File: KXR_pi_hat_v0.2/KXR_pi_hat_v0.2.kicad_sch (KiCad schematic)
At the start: 6 parts, among them J1 Conn_01x05_Pin, J2 Conn_01x05_Pin, J3 Conn_01x05_Pin, J4 Conn_01x05_Pin, U2 Raspberry_Pi_2_3

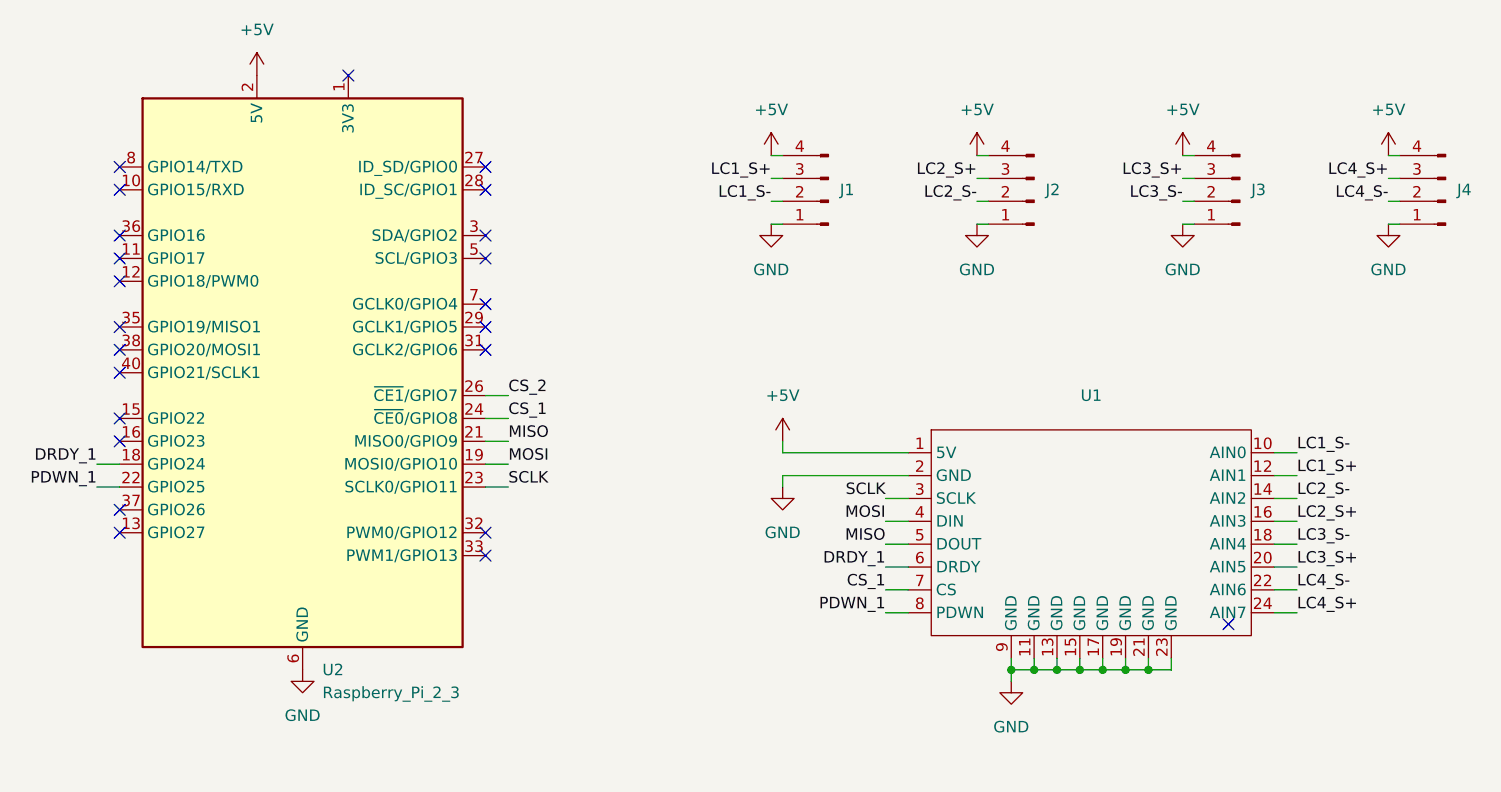
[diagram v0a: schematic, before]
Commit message: Finishing touches and production files
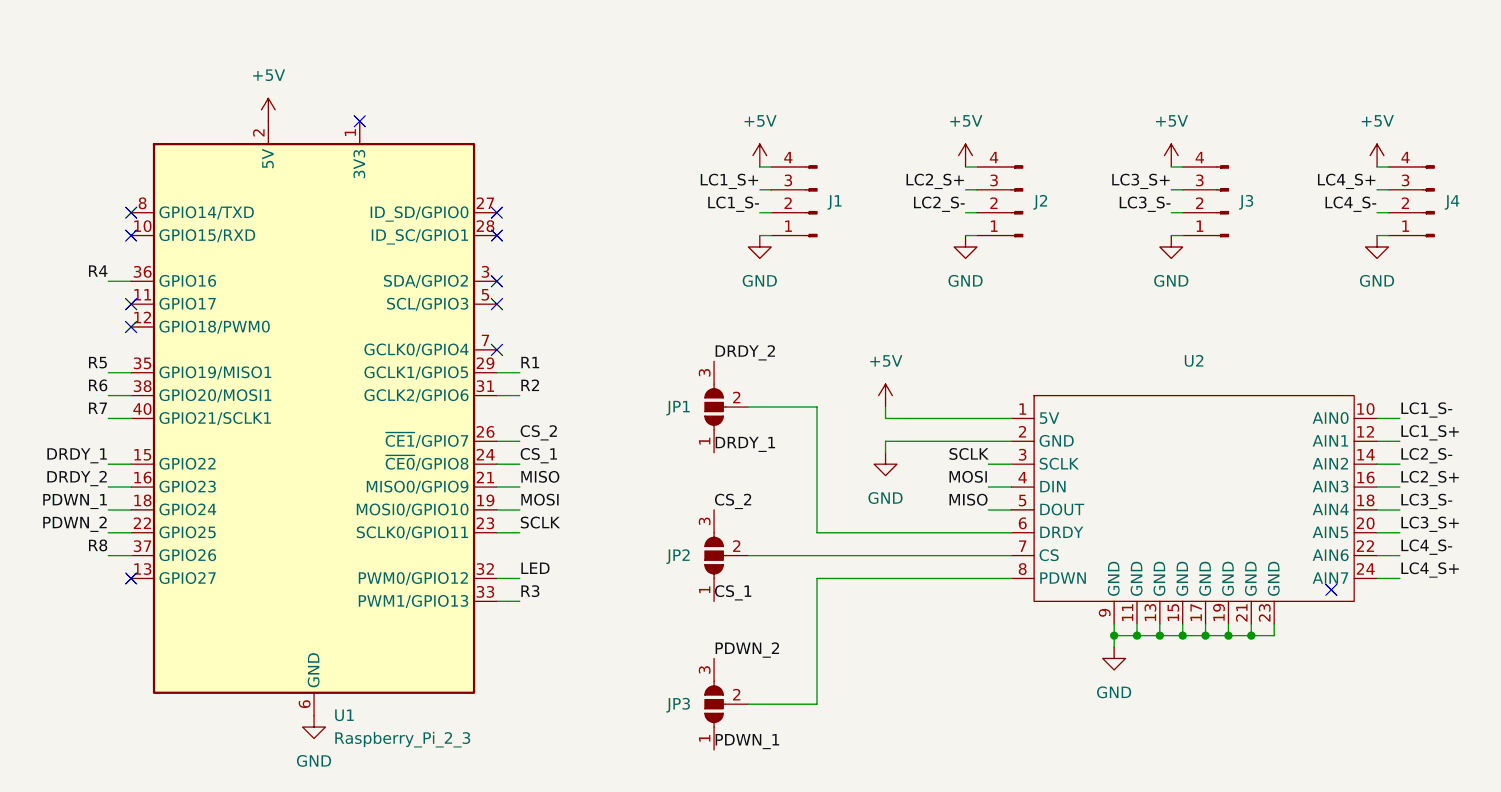
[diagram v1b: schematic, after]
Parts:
- added JP1, JP2, JP3: SolderJumper_3_Open, Jumper:SolderJumper-3_P1.3mm_Open_RoundedPad1.0x1.5mm_NumberLabels, symbol Jumper:SolderJumper_3_Open
- renumbered U2 to U1, U1 to U2
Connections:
- net CS_1: now also JP2.1 (A); no longer U2.7 (CS)
- net CS_2: now also JP2.3 (B)
- net DRDY_1: now also U1.15 (GPIO22), JP1.1 (A); no longer U1.18 (GPIO24), U2.6 (DRDY)
- net PDWN_1: now also U1.18 (GPIO24), JP3.1 (A); no longer U1.22 (GPIO25), U2.8 (PDWN)
- net DRDY_2: now reaches U1.16 (GPIO23)
- net DRDY_2: now also JP1.3 (B)
- net R1: now reaches U1.29 (GCLK1/GPIO5)
- net R2: now reaches U1.31 (GCLK2/GPIO6)
- net LED: now reaches U1.32 (PWM0/GPIO12)
- net R3: now reaches U1.33 (PWM1/GPIO13)
- net R5: now reaches U1.35 (GPIO19/MISO1)
- net R4: now reaches U1.36 (GPIO16)
- net R8: now reaches U1.37 (GPIO26)
- net R6: now reaches U1.38 (GPIO20/MOSI1)
- net R7: now reaches U1.40 (GPIO21/SCLK1)
- new net: JP2.2 (C), U2.7 (CS)
- new net: JP3.2 (C), U2.8 (PDWN)
- new net: JP1.2 (C), U2.6 (DRDY)
- new net PDWN_2: JP3.3 (B), U1.22 (GPIO25)
- no-connect marks 23 -> 12
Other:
- moved on the sheet: J1, J2, J3, J4, U1, U2
